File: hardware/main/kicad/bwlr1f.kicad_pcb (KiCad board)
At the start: 4 copper layers, 61.2 x 26.1 mm, 69 parts, among them J1 Conn_01x02, U1 RAK3172-SIP, U2 NBM7100ABQX, U3 ZD24C08A, U4 BME688, U5 RV-3028-C7

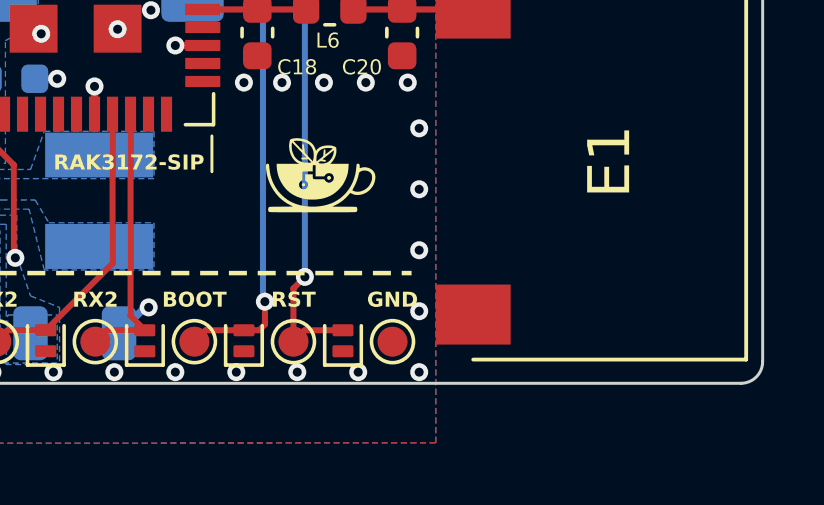
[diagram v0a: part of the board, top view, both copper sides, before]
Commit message: Update for Programmer
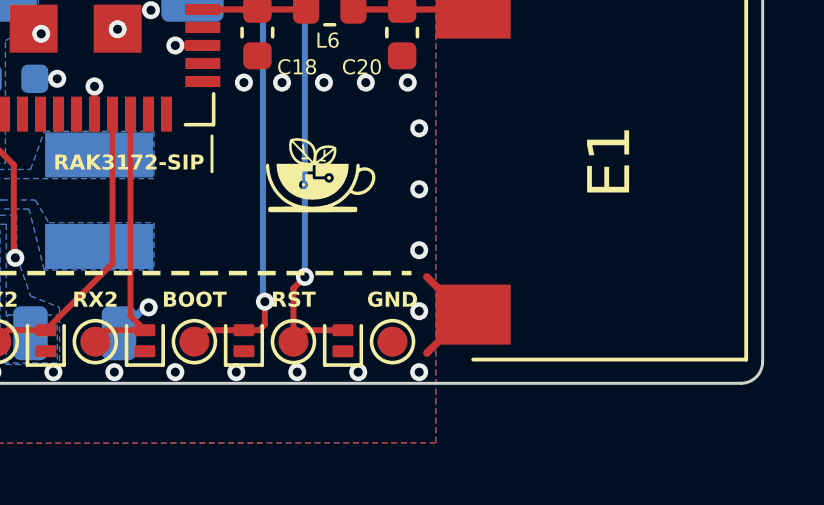
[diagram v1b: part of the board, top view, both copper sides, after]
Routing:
- net GND: track 28.2 -> 32.4 mm
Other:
- board text added: "Dimension @User.2"
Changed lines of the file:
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@@
 		)
 	)
+	(gr_text "Dimension @User.2"
+		(at 105.469999 126.303 0)
+		(layer "User.2")
+		(effects
+			(font
+				(size 1 1)
+				(thickness 0.15)
+			)
+			(justify left bottom)
+		)
+	)
 	(dimension
 		(type aligned)
 		(layer "User.2")
 		(pts
-			(xy 107.869999 97.489999) (xy 107.869999 123.62)
+			(xy 165.981847 99.257376) (xy 165.981847 121.84911)
 		)
-		(height -63.132)
-		(gr_text "26,1300 mm"
-			(at 169.851999 110.555 90)
+		(height -4.004152)
+		(gr_text "22,5917 mm"
+			(at 171.001999 110.555 90)
 			(layer "User.2")
 			(effects
@@
 			(thickness 0.15)
 			(arrow_length 1.27)
-			(text_position_mode 0)
+			(text_position_mode 2)
 			(extension_height 0.58642)
 			(extension_offset 0.5) keep_text_aligned)
@@
 			(xy 105.469999 110.555) (xy 166.702471 110.553)
 		)
-		(height -23.799694)
+		(height -16.394027)
 		(gr_text "61,2325 mm"
-			(at 136.08542 85.604306 0.001871418142)
+			(at 136.085662 93.009973 0.001871418142)
+			(layer "User.2")
+			(effects
+				(font
+					(size 1 1)
+					(thickness 0.15)
+				)
+			)
+		)
+		(format
+			(prefix "")
+			(suffix "")
+			(units 3)
+			(units_format 1)
+			(precision 4)
+		)
+		(style
+			(thickness 0.15)
+			(arrow_length 1.27)
+			(text_position_mode 0)
+			(extension_height 0.58642)
+			(extension_offset 0.5) keep_text_aligned)
+	)
+	(dimension
+		(type aligned)
+		(layer "User.2")
+		(pts
+			(xy 107.869999 97.489999) (xy 107.869999 123.62)
+		)
+		(height 5.447999)
+		(gr_text "26,1300 mm"
+			(at 101.272 110.555 90)
 			(layer "User.2")
 			(effects
@@
 	)
 	(segment
+		(start 156.763999 119.558)
+		(end 155.507999 118.302)
+		(width 0.25)
+		(layer "F.Cu")
+		(net 1)
+	)
+	(segment
 		(start 151.688999 103.763)
 		(end 151.697999 103.754)
@@
 	)
 	(segment
+		(start 156.791999 119.558)
+		(end 155.507999 120.842)
+		(width 0.25)
+		(layer "F.Cu")
+		(net 1)
+	)
+	(segment
+		(start 157.053999 119.558)
+		(end 156.763999 119.558)
+		(width 0.25)
+		(layer "F.Cu")
+		(net 1)
+	)
+	(segment
 		(start 134.270999 105.884)
 		(end 133.790999 105.884)
@@
 	)
 	(segment
+		(start 157.053999 119.558)
+		(end 156.791999 119.558)
+		(width 0.25)
+		(layer "F.Cu")
+		(net 1)
+	)
+	(segment
 		(start 147.125999 110.588)
 		(end 148.041847 110.588)
@@
 		(layers "F.Cu" "In1.Cu" "In2.Cu" "B.Cu")
 		(hatch edge 0.5)
-		(connect_pads yes
+		(connect_pads
 			(clearance 0.2)
 		)
@@
 		(filled_areas_thickness no)
 		(fill yes
-			(thermal_gap 0.5)
-			(thermal_bridge_width 0.5)
+			(thermal_gap 0.2)
+			(thermal_bridge_width 0.2)
 		)
 		(polygon

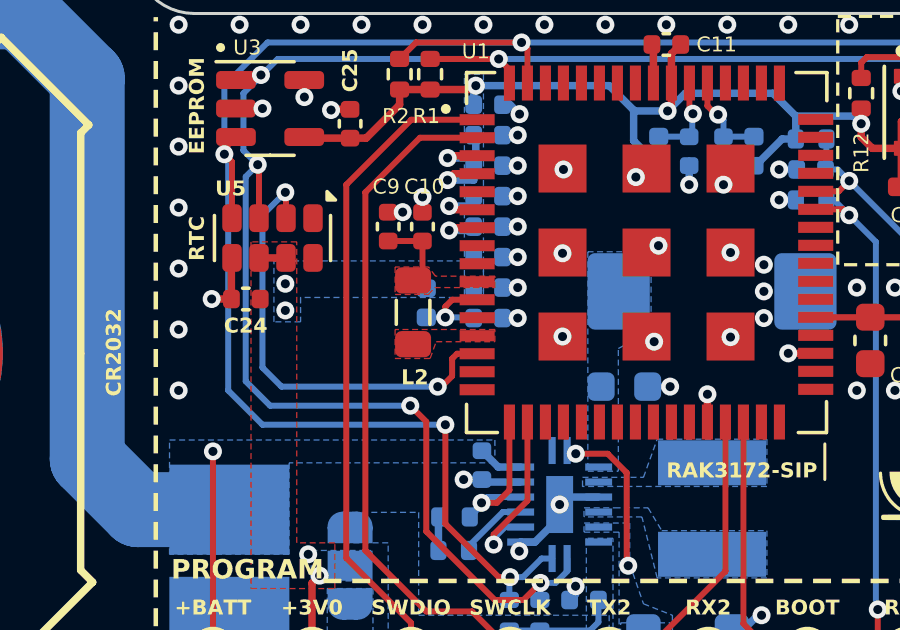
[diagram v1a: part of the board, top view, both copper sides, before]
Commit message: Finish Production File for Main Board
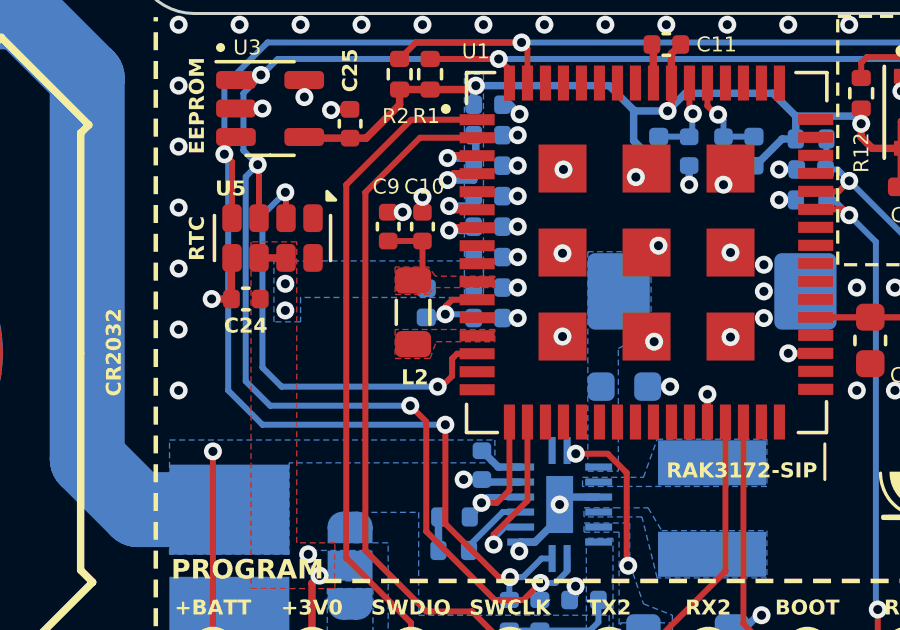
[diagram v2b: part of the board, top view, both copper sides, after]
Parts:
- TP1: value 3V0 -> 90055-AS
- TP2: value BATT+ -> 90055-AS
- TP3: value RX2 -> 90055-AS
- TP4: value TX2 -> 90055-AS
- TP5: value SWCLK -> 90055-AS
- TP6: value SWDIO -> 90055-AS
- TP7: value RST -> 90055-AS
- TP8: value BOOT -> 90055-AS
- TP9: value GND -> 90055-AS
